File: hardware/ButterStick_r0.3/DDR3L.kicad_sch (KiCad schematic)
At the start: 2 parts, among them U4 MT41K64M16TW-107_J-TR

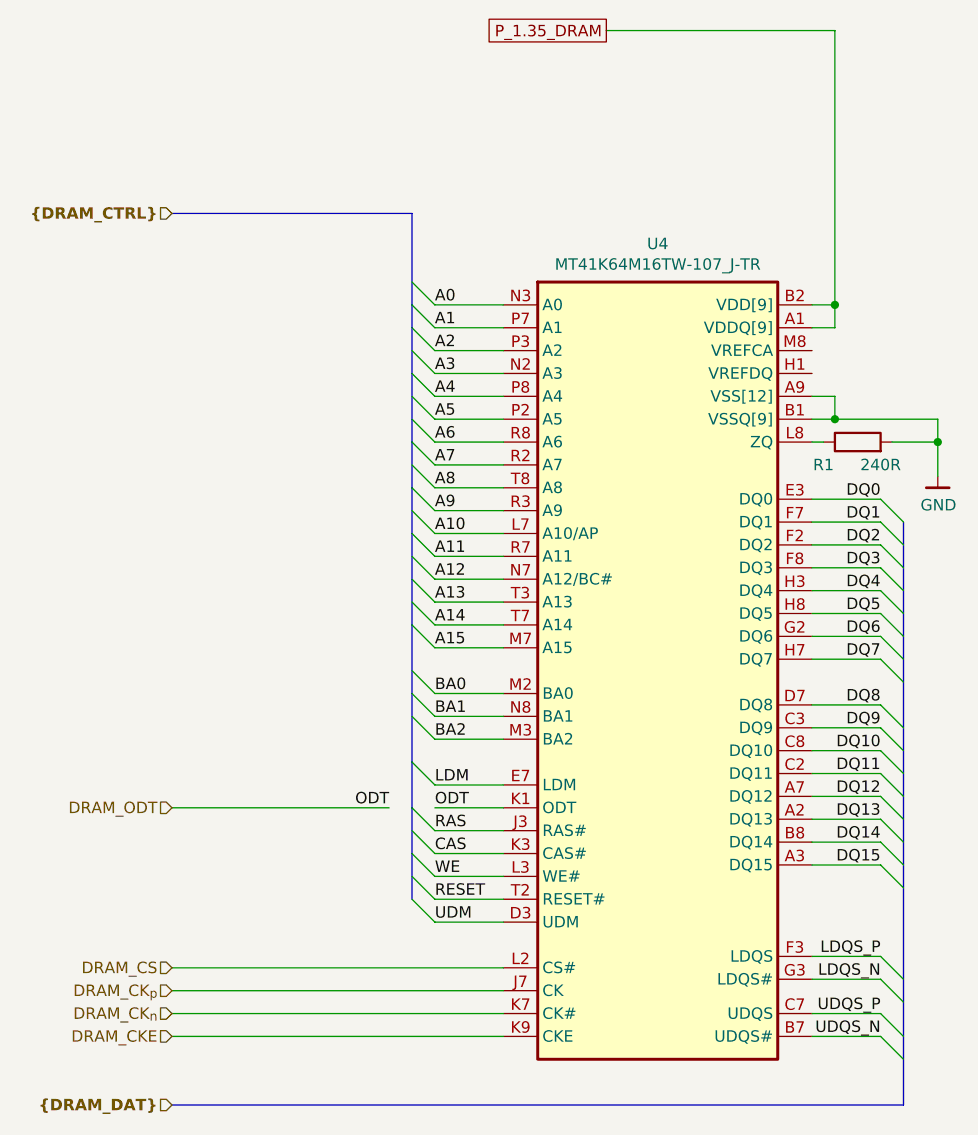
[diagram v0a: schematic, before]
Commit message: hw.r0_3: major blocks roughly routed
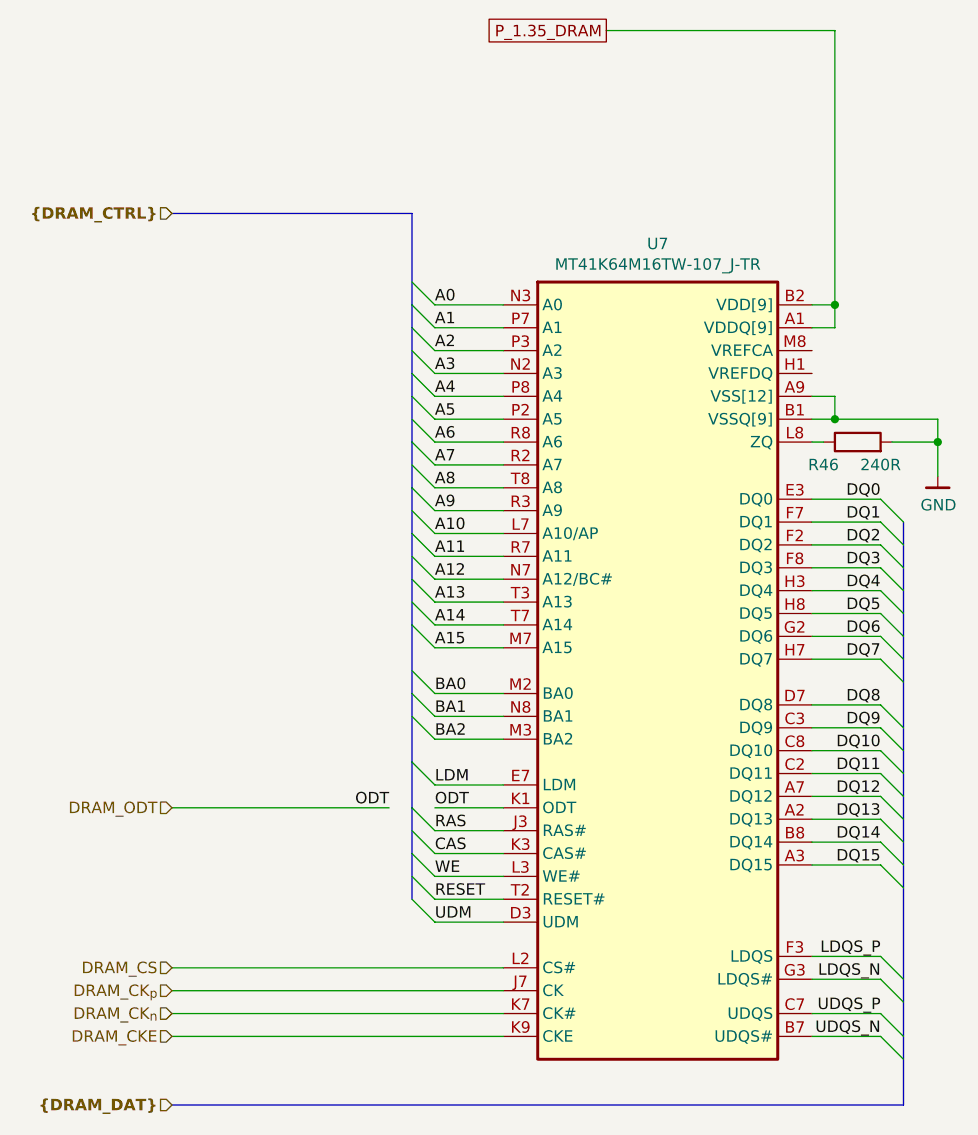
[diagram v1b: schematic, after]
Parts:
- renumbered R1 to R46, U4 to U7
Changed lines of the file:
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@@
   (bus (pts (xy 110.49 66.04) (xy 110.49 68.58)))
   (bus (pts (xy 110.49 68.58) (xy 110.49 73.66)))
-  (bus (pts (xy 110.49 73.66) (xy 110.49 78.74)))
-  (bus (pts (xy 110.49 78.74) (xy 110.49 81.28)))
+  (bus (pts (xy 110.49 73.66) (xy 110.49 76.2)))
+  (bus (pts (xy 110.49 76.2) (xy 110.49 81.28)))
   (bus (pts (xy 110.49 81.28) (xy 110.49 86.36)))
   (bus (pts (xy 110.49 86.36) (xy 110.49 91.44)))
@@
   (bus (pts (xy 165.1 107.95) (xy 165.1 115.57)))
   (bus (pts (xy 165.1 115.57) (xy 165.1 120.65)))
-  (bus (pts (xy 165.1 120.65) (xy 165.1 125.73)))
-  (bus (pts (xy 165.1 125.73) (xy 165.1 128.27)))
+  (bus (pts (xy 165.1 120.65) (xy 165.1 123.19)))
+  (bus (pts (xy 165.1 123.19) (xy 165.1 128.27)))
   (bus (pts (xy 165.1 128.27) (xy 165.1 140.97)))
   (bus (pts (xy 165.1 140.97) (xy 165.1 143.51)))
@@
   )
   (symbol (lib_id "power:GND") (at 168.91 85.09 0)
-    (property "Reference" "#PWR0224" (id 0) (at 168.91 91.44 0)
+    (property "Reference" "#PWR083" (id 0) (at 168.91 91.44 0)
       (effects (font (size 1.27 1.27)) hide)
     )
@@
   )
   (symbol (lib_id "Device:R") (at 160.02 81.28 90)
-    (property "Reference" "R1" (id 0) (at 156.21 83.82 90))
+    (property "Reference" "R46" (id 0) (at 156.21 83.82 90))
     (property "Value" "240R" (id 1) (at 162.56 83.82 90))
     (property "Footprint" "" (id 2) (at 160.02 83.058 90)
@@
   )
   (symbol (lib_id "gkl_mem:MT41K512M16TW") (at 137.16 96.52 0)
-    (property "Reference" "U4" (id 0) (at 137.795 59.2582 0))
+    (property "Reference" "U7" (id 0) (at 137.795 59.2582 0))
     (property "Value" "MT41K64M16TW-107_J-TR" (id 1) (at 137.795 61.5442 0))
     (property "Footprint" "Package_BGA:BGA-96_9.0x13.0mm_Layout2x3x16_P0.8mm" (id 2) (at 138.43 58.42 0)
